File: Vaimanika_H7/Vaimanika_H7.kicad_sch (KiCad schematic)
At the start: 67 parts, among them J1 USB_C_Receptacle_USB2.0_16P, J2 Conn_01x08, J3 Conn_01x08, J4 +VLIPO, J5 GND, J6 Conn_01x08, J7 Conn_01x03, Q1 AO3400A, Q2 AO3401A, U1 TPS54302, U2 TPS54302, U3 USBLC6-2P6

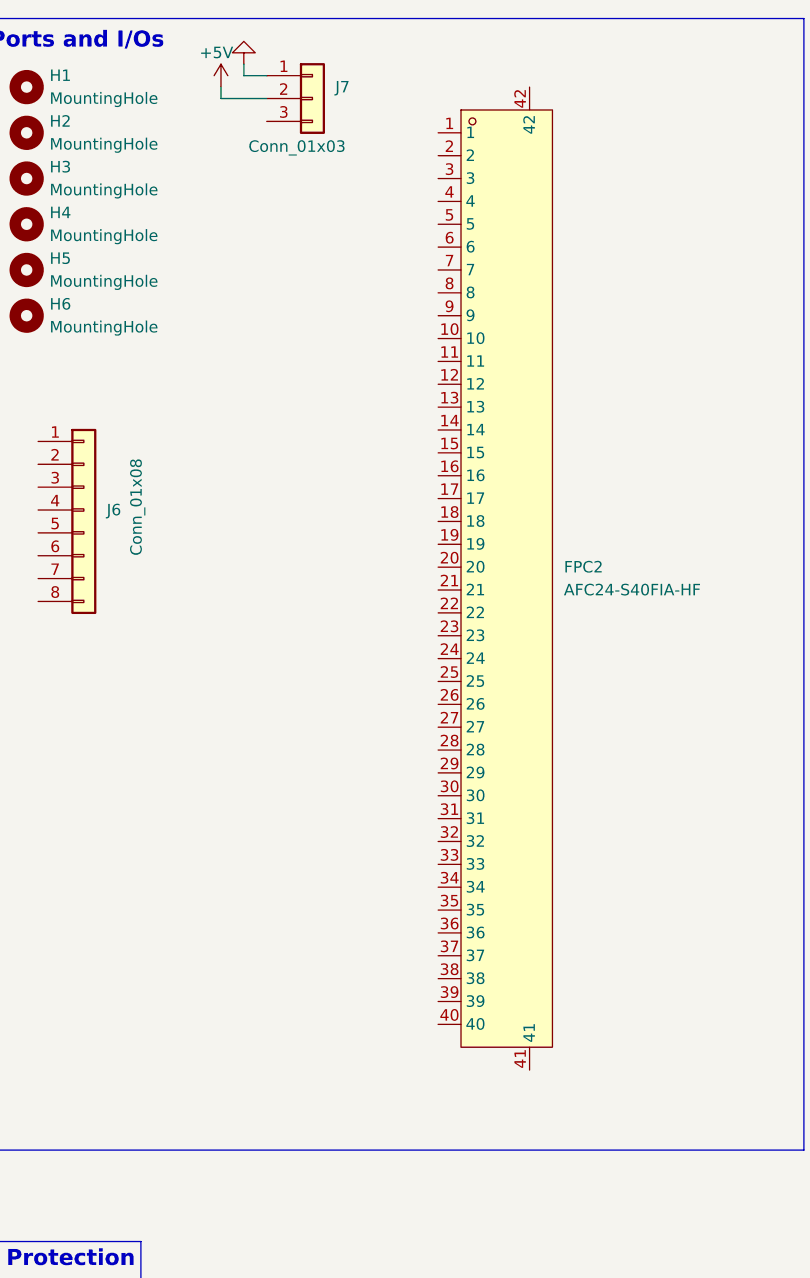
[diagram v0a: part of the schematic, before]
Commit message: 23-04-2026
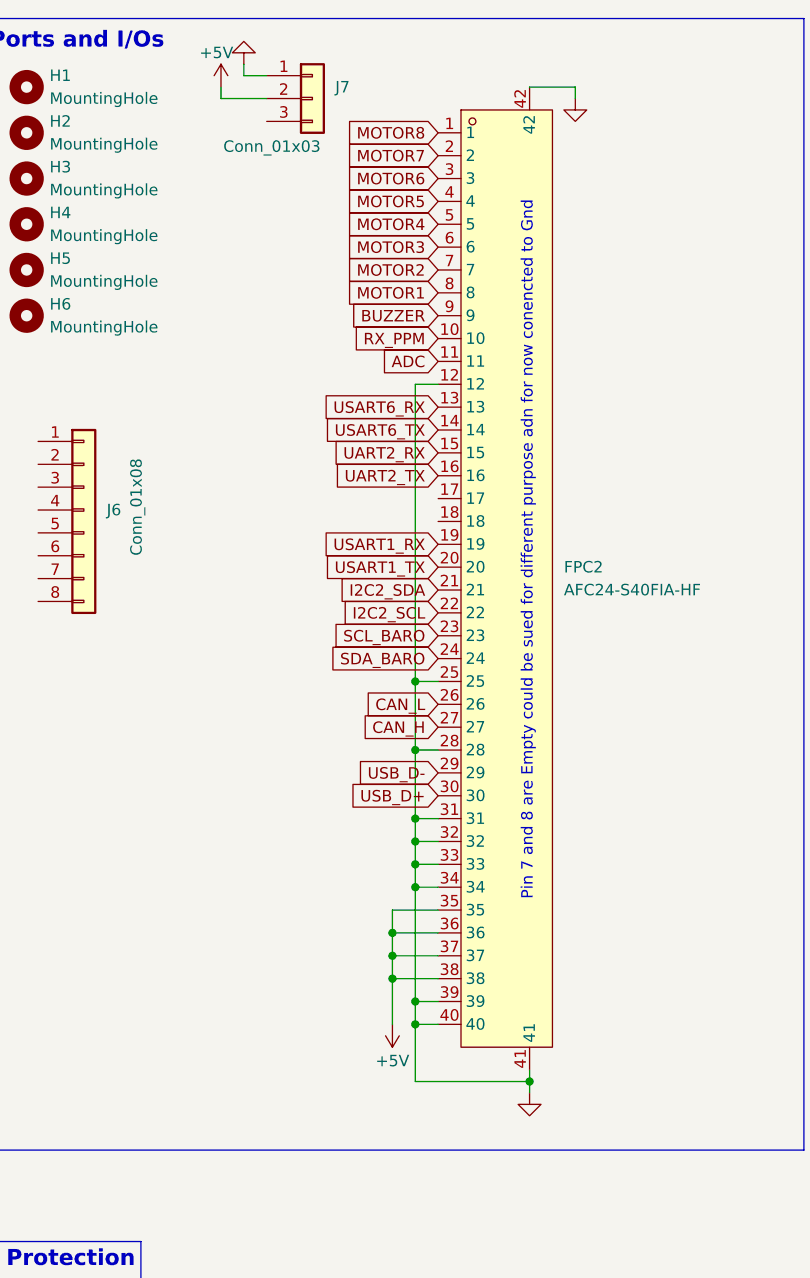
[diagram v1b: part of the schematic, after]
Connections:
- net +5V: now also FPC2.35, FPC2.36, FPC2.37, FPC2.38
- net BUZZER: now also FPC2.9
- net GND: now also FPC2.12, FPC2.25, FPC2.28, FPC2.31, FPC2.32, FPC2.33, FPC2.34, FPC2.39, FPC2.40, FPC2.41, FPC2.42
- net USB_D+: now also FPC2.30
- net USB_D-: now also FPC2.29
- net MOTOR8: now reaches FPC2.1
- net RX_PPM: now reaches FPC2.10
- net ADC: now reaches FPC2.11
- net USART6_RX: now reaches FPC2.13
- net USART6_TX: now reaches FPC2.14
- net UART2_RX: now reaches FPC2.15
- net UART2_TX: now reaches FPC2.16
- net USART1_RX: now reaches FPC2.19
- net MOTOR7: now reaches FPC2.2
- net USART1_TX: now reaches FPC2.20
- net I2C2_SDA: now reaches FPC2.21
- net I2C2_SCL: now reaches FPC2.22
- net SCL_BARO: now reaches FPC2.23
- net SDA_BARO: now reaches FPC2.24
- net CAN_L: now reaches FPC2.26
- net CAN_H: now reaches FPC2.27
- net MOTOR6: now reaches FPC2.3
- net MOTOR5: now reaches FPC2.4
- net MOTOR4: now reaches FPC2.5
- net MOTOR3: now reaches FPC2.6
- net MOTOR2: now reaches FPC2.7
- net MOTOR1: now reaches FPC2.8
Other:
- note added: "Pin 7 and 8 are Empty could be sued for different purpose adn for now conencted to Gnd"
